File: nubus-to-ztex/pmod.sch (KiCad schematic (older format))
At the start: 2 parts, among them J8 SMH-108-02-L-D (Pmod 2x8 F)

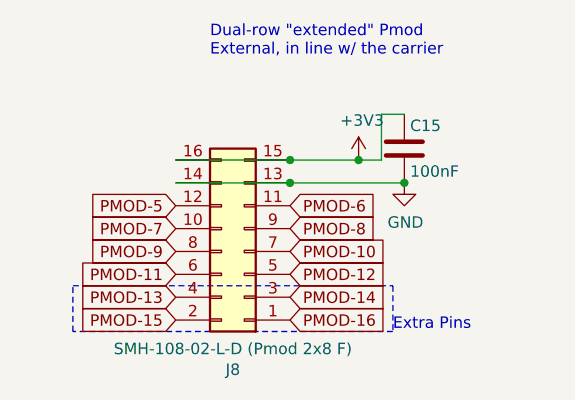
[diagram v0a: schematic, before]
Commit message: some BoM optimization
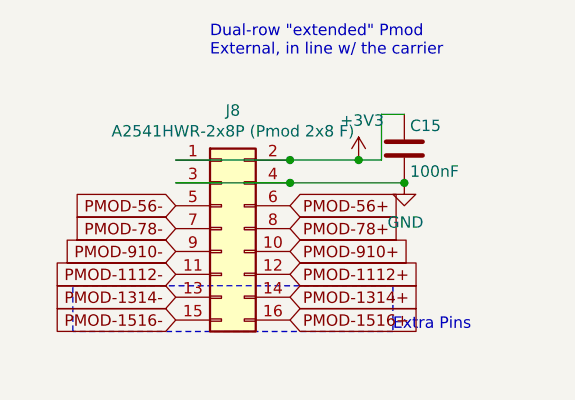
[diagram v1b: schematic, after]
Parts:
- C15: MPN CC0603KRX7R8BB104 -> CC0603KRX7R9BB104; URL https://www.lcsc.com/product-detail/Multilayer-Ceramic-Capacitors-MLCC-SMD-SMT_YAGEO-CC0603KRX7R8BB104_C92490.html -> https://www.lcsc.com/product-detail/Multilayer-Ceramic-Capacitors-MLCC-SMD-SMT_YAGEO-CC0603KRX7R9BB104_C14663.html
- J8: value SMH-108-02-L-D (Pmod 2x8 F) -> A2541HWR-2x8P (Pmod 2x8 F); footprint For_SeeedStudio:SAMTEC-SMH-108-02-X-D -> For_SeeedStudio:PinSocket_2x08_P2.54mm_Horizontal_ForSeeedStudio; MPN SMH-108-02-L-D -> A2541HWR-2x8P; URL https://www.mouser.fr/ProductDetail/Samtec/SMH-108-02-L-D?q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 -> https://www.lcsc.com/product-detail/Female-Headers_CJT-Chan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
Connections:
- net PMOD-13 is gone; now on net GND: J8.4 (Pin_4)
- net PMOD-14 is gone; now on net GND: J8.3 (Pin_3)
- net PMOD-15 is gone; now on net +3V3: J8.2 (Pin_2)
- net PMOD-16 is gone; now on net +3V3: J8.1 (Pin_1)
- net +3V3: no longer J8.15 (Pin_15), J8.16 (Pin_16)
- net GND: no longer J8.13 (Pin_13), J8.14 (Pin_14)
- net PMOD-10 renamed PMOD-78-
- net PMOD-11 renamed PMOD-56+
- net PMOD-12 renamed PMOD-56-
- net PMOD-5 renamed PMOD-1112+
- net PMOD-6 renamed PMOD-1112-
- net PMOD-7 renamed PMOD-910+
- net PMOD-8 renamed PMOD-910-
- net PMOD-9 renamed PMOD-78+
- new net PMOD-1314+: J8.14 (Pin_14)
- new net PMOD-1314-: J8.13 (Pin_13)
- new net PMOD-1516+: J8.16 (Pin_16)
- new net PMOD-1516-: J8.15 (Pin_15)
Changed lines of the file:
@@
 L Connector_Generic:Conn_02x08_Odd_Even J8
 U 1 1 63467144
-P 7450 3700
-F 0 "J8" H 7500 4217 50  0000 C CNN
-F 1 "SMH-108-02-L-D (Pmod 2x8 F)" H 7500 4126 50  0000 C CNN
-F 2 "For_SeeedStudio:SAMTEC-SMH-108-02-X-D" H 7450 3700 50  0001 C CNN
-F 3 "~" H 7450 3700 50  0001 C CNN
-F 4 "SMH-108-02-L-D" H 7450 3700 50  0001 C CNN "MPN"
-F 5 "https://www.mouser.fr/ProductDetail/Samtec/SMH-108-02-L-D?qs=%252BZP6%2F%252BtExtAyrMiVCu9Apg%3D%3D" H 7450 3700 50  0001 C CNN "URL"
-	1    7450 3700
-	-1   0    0    1
+P 7350 3600
+F 0 "J8" H 7400 4117 50  0000 C CNN
+F 1 "A2541HWR-2x8P (Pmod 2x8 F)" H 7400 4026 50  0000 C CNN
+F 2 "For_SeeedStudio:PinSocket_2x08_P2.54mm_Horizontal_ForSeeedStudio" H 7350 3600 50  0001 C CNN
+F 3 "~" H 7350 3600 50  0001 C CNN
+F 4 "A2541HWR-2x8P" H 7350 3600 50  0001 C CNN "MPN"
+F 5 "https://www.lcsc.com/product-detail/Female-Headers_CJT-Changjiang-Connectors-A2541HWR-2x8P_C239359.html" H 7350 3600 50  0001 C CNN "URL"
+	1    7350 3600
+	1    0    0    -1
 $EndComp
 Text GLabel 7150 3500 0    50   Input ~ 0
-PMOD-5
+PMOD-56-
 Text GLabel 7150 3600 0    50   Input ~ 0
-PMOD-7
+PMOD-78-
 Text GLabel 7150 3700 0    50   Input ~ 0
-PMOD-9
+PMOD-910-
 Text GLabel 7150 3800 0    50   Input ~ 0
-PMOD-11
+PMOD-1112-
 Text GLabel 7650 3800 2    50   Input ~ 0
-PMOD-12
+PMOD-1112+
 Text GLabel 7650 3500 2    50   Input ~ 0
-PMOD-6
+PMOD-56+
 Text GLabel 7650 3600 2    50   Input ~ 0
-PMOD-8
+PMOD-78+
 Text GLabel 7650 3700 2    50   Input ~ 0
-PMOD-10
+PMOD-910+
 $Comp
 L power:GND #PWR0151
@@
 F 3 "" H 8150 3250 50  0000 C CNN
 F 4 "www.yageo.com" H 8150 3250 50  0001 C CNN "MNF1_URL"
-F 5 "CC0603KRX7R8BB104" H 8150 3250 50  0001 C CNN "MPN"
+F 5 "CC0603KRX7R9BB104" H 8150 3250 50  0001 C CNN "MPN"
 F 6 "603-CC603KRX7R8BB104" H 8150 3250 50  0001 C CNN "Mouser"
 F 7 "?" H 8150 3250 50  0001 C CNN "Digikey"
@@
 F 9 "?" H 8150 3250 50  0001 C CNN "Koncar"
 F 10 "TB" H 8150 3250 50  0001 C CNN "Side"
-F 11 "https://www.lcsc.com/product-detail/Multilayer-Ceramic-Capacitors-MLCC-SMD-SMT_YAGEO-CC0603KRX7R8BB104_C92490.html" H 3000 6050 50  0001 C CNN "URL"
+F 11 "https://www.lcsc.com/product-detail/Multilayer-Ceramic-Capacitors-MLCC-SMD-SMT_YAGEO-CC0603KRX7R9BB104_C14663.html" H 3000 6050 50  0001 C CNN "URL"
 	1    8150 3250
 	1    0    0    -1
@@
 	8050 3100 8150 3100
 Text GLabel 7650 3900 2    50   Input ~ 0
-PMOD-14
+PMOD-1314+
 Text GLabel 7650 4000 2    50   Input ~ 0
-PMOD-16
+PMOD-1516+
 Text GLabel 7150 3900 0    50   Input ~ 0
-PMOD-13
+PMOD-1314-
 Text GLabel 7150 4000 0    50   Input ~ 0
-PMOD-15
+PMOD-1516-
 Wire Notes Line
 	6700 3850 8100 3850
@@
 Text Notes 8100 4050 0    50   ~ 0
 Extra Pins
+Connection ~ 7950 3300
+Connection ~ 8150 3400
+Wire Wire Line
+	7650 3300 7950 3300
+Wire Wire Line
+	7650 3400 8150 3400
 Wire Wire Line
 	7150 3300 7650 3300
-Wire Wire Line
-	7650 3300 7950 3300
 Connection ~ 7650 3300
-Connection ~ 7950 3300
 Wire Wire Line
 	7150 3400 7650 3400
-Wire Wire Line
-	7650 3400 8150 3400
 Connection ~ 7650 3400
-Connection ~ 8150 3400
 $EndSCHEMATC
